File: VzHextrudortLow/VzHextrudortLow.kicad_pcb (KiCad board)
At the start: 2 copper layers, 50.6 x 38 mm, 12 parts, among them J1 Conn_01x04, J12 Conn_01x02, J2 Conn_01x05, J3 Conn_01x04, J4 Conn_02x10_Top_Bottom, J5 Conn_01x02, J6 Conn_01x03, J7 Conn_01x05, J9 Conn_01x02

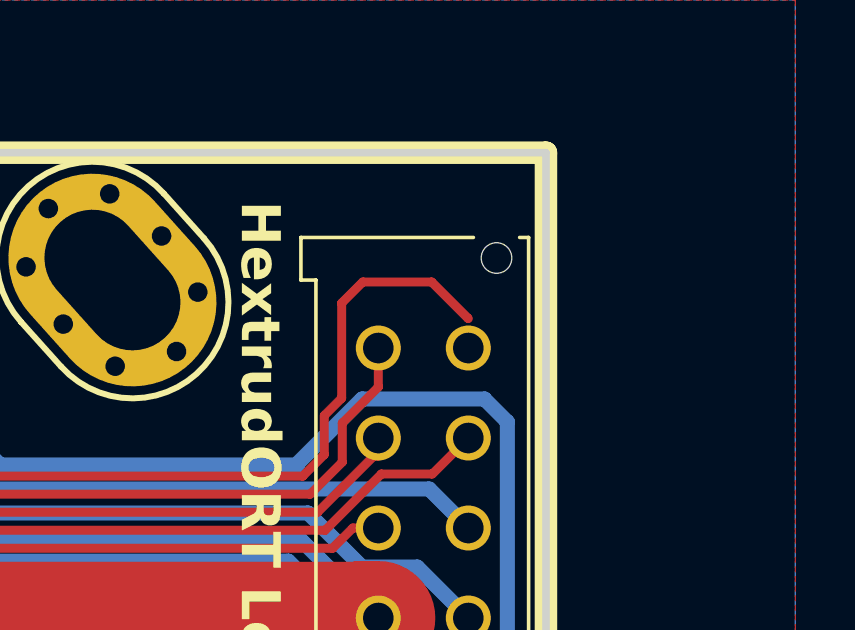
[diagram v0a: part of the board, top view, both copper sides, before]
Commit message: Add files via upload
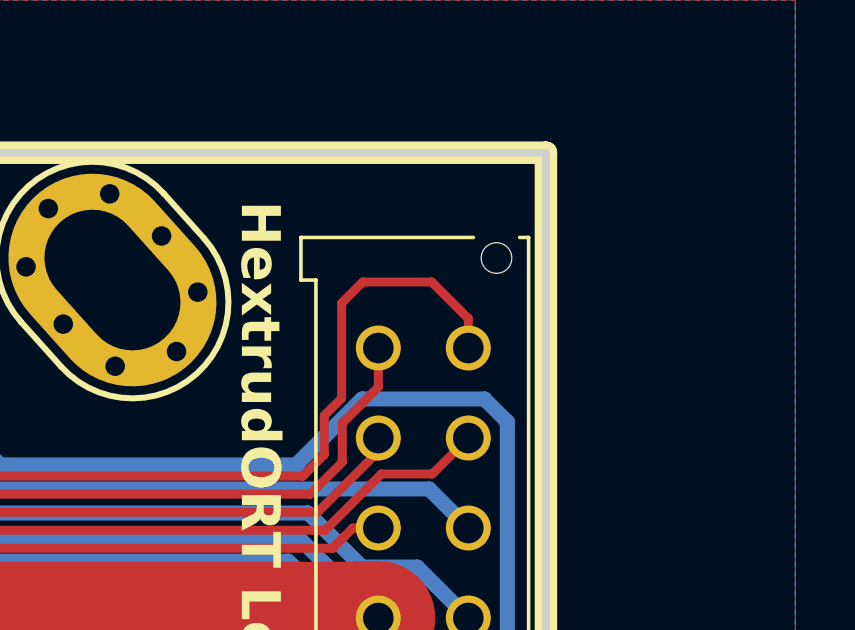
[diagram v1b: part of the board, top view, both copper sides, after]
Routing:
- net /FIL_SENS: track 40.7 -> 41.6 mm
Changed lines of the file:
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@@
 	)
 	(segment
-		(start 142.671 95.171)
-		(end 165.580704 95.171)
+		(start 166.879 89.402529)
+		(end 167.582529 88.699)
+		(width 0.3)
+		(layer "F.Cu")
+		(net 12)
+	)
+	(segment
+		(start 166.298 94.453704)
+		(end 166.298 93.153587)
 		(width 0.3)
 		(layer "F.Cu")
@@
 	)
 	(segment
-		(start 166.879 89.402529)
-		(end 167.582529 88.699)
-		(width 0.3)
-		(layer "F.Cu")
-		(net 12)
-	)
-	(segment
 		(start 169.879 88.699)
-		(end 171.08 89.9)
-		(width 0.3)
-		(layer "F.Cu")
-		(net 12)
-	)
-	(segment
-		(start 171.08 89.9)
 		(end 171.1 89.92)
 		(width 0.3)
@@
 	)
 	(segment
-		(start 166.298 93.153587)
-		(end 166.879 92.572587)
+		(start 167.582529 88.699)
+		(end 169.879 88.699)
+		(width 0.3)
+		(layer "F.Cu")
+		(net 12)
+	)
+	(segment
+		(start 142.671 95.171)
+		(end 165.580704 95.171)
+		(width 0.3)
+		(layer "F.Cu")
+		(net 12)
+	)
+	(segment
+		(start 171.1 89.92)
+		(end 171.1 90.9)
+		(width 0.3)
+		(layer "F.Cu")
+		(net 12)
+	)
+	(segment
+		(start 166.879 92.572587)
+		(end 166.879 89.402529)
 		(width 0.3)
 		(layer "F.Cu")
@@
 		(start 139.926 93.576057)
 		(end 141.048943 94.699)
-		(width 0.3)
-		(layer "F.Cu")
-		(net 12)
-	)
-	(segment
-		(start 165.580704 95.171)
-		(end 166.298 94.453704)
 		(width 0.3)
 		(layer "F.Cu")
@@
 	)
 	(segment
-		(start 167.582529 88.699)
-		(end 169.879 88.699)
+		(start 165.580704 95.171)
+		(end 166.298 94.453704)
 		(width 0.3)
 		(layer "F.Cu")
@@
 	)
 	(segment
-		(start 166.879 92.572587)
-		(end 166.879 89.402529)
+		(start 166.298 93.153587)
+		(end 166.879 92.572587)
 		(width 0.3)
 		(layer "F.Cu")
-		(net 12)
-	)
-	(segment
-		(start 166.298 94.453704)
-		(end 166.298 93.153587)
-		(width 0.3)
-		(layer "F.Cu")
